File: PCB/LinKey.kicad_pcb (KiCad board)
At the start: 2 copper layers, 25 x 43.5 mm, 1 part

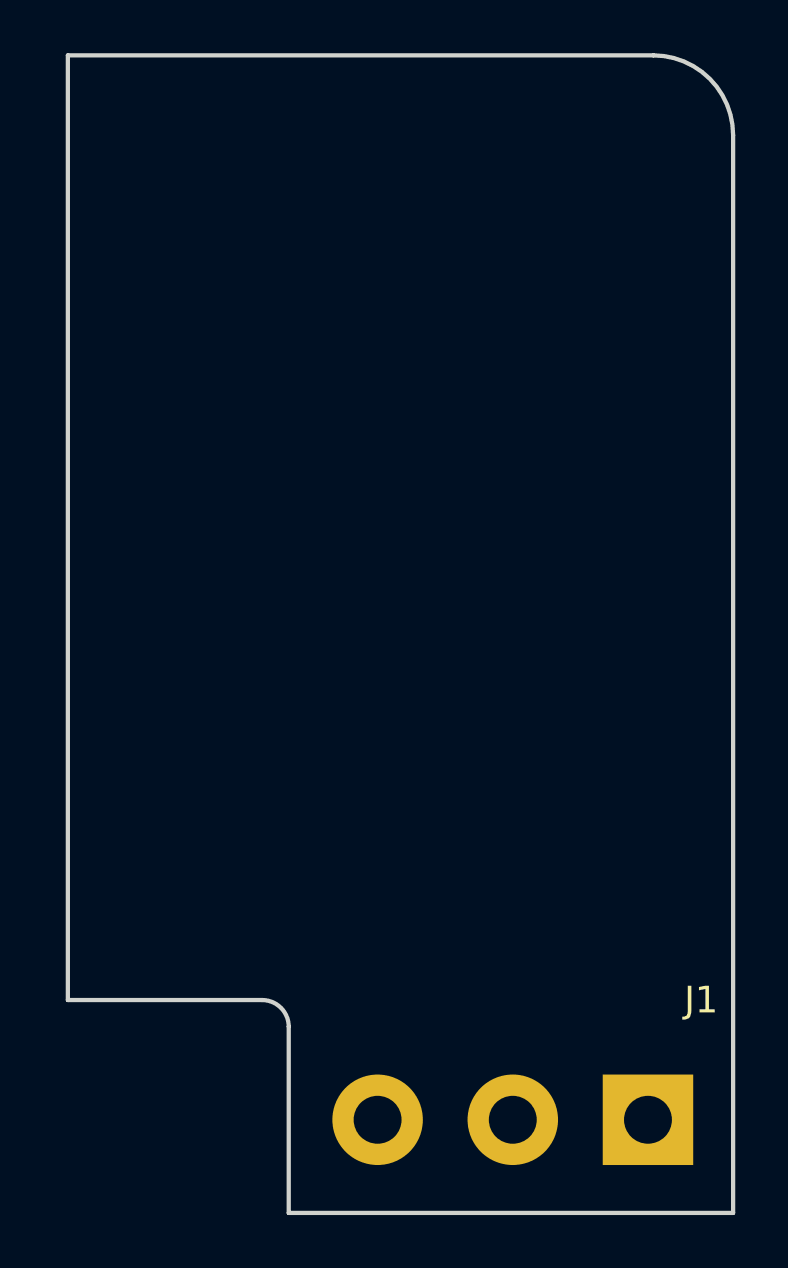
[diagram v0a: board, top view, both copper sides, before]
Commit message: Release PCB v1
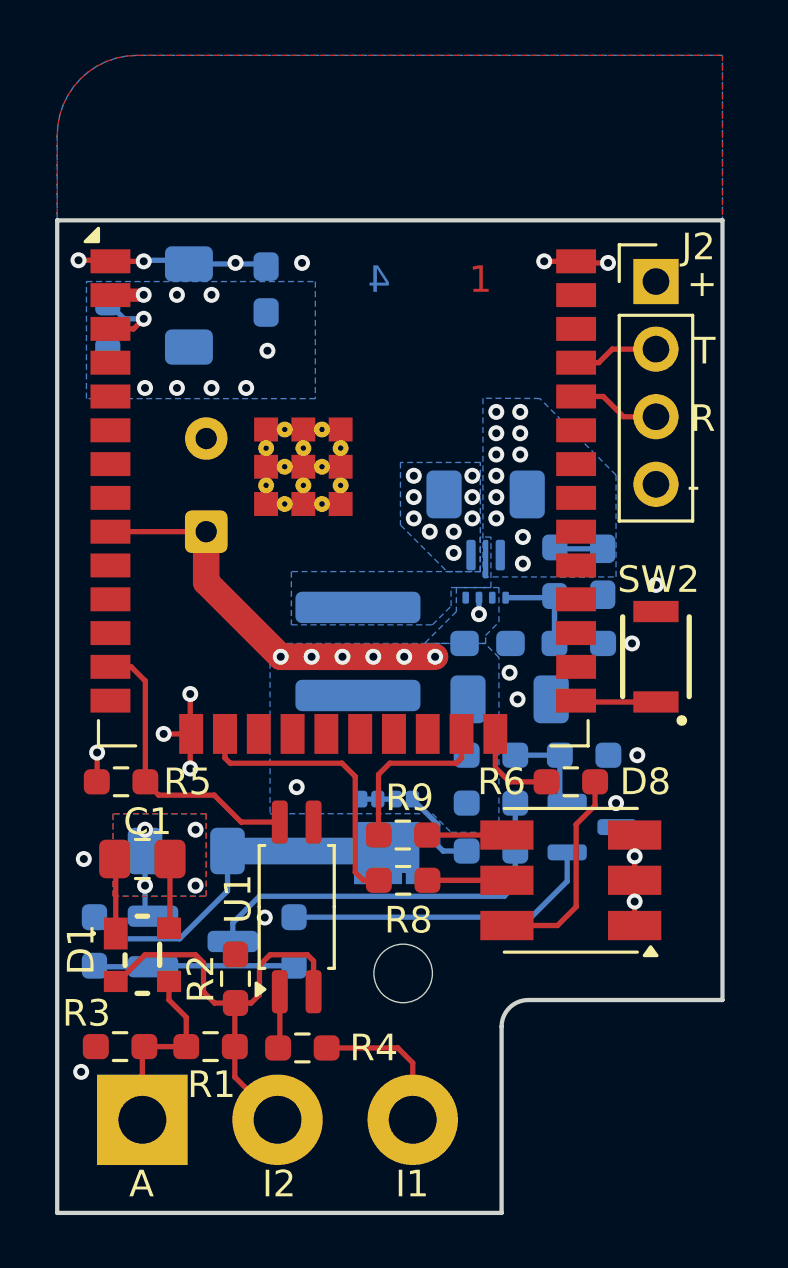
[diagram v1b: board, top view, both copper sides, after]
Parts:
- added C1: 2,2u, Capacitor_SMD:C_0805_2012Metric_Pad1.18x1.45mm_HandSolder, F.Cu at (144.5, 86.2)
- added C2: 1F, Capacitor_THT:CP_Radial_D8.0mm_P3.50mm, B.Cu at (146.9, 73.9)
- added C3: 22u, Capacitor_SMD:C_1206_3216Metric_Pad1.33x1.80mm_HandSolder, B.Cu at (158.3, 80.2)
- added C4: 100n, Capacitor_SMD:C_0603_1608Metric_Pad1.08x0.95mm_HandSolder, B.Cu at (157.5, 78.1)
- added C5: 175p, Capacitor_SMD:C_0603_1608Metric_Pad1.08x0.95mm_HandSolder, B.Cu at (161.8, 75.4)
- added C6: 22u, Capacitor_SMD:C_1206_3216Metric_Pad1.33x1.80mm_HandSolder, B.Cu at (157.4, 72.5)
- added C7: 22u, Capacitor_SMD:C_1206_3216Metric_Pad1.33x1.80mm_HandSolder, B.Cu at (146.2, 65.4)
- added C8: 100n, Capacitor_SMD:C_0603_1608Metric_Pad1.08x0.95mm_HandSolder, B.Cu at (149.2, 64.8)
- added D1: BAS_4002A_RPP_E6327, LinKey_Lib_Footprints:BAS4002ARPPE6327, F.Cu at (144.5, 89.8)
- added D8: LED_RGB, LED_SMD:LED_RGB_5050-6, F.Cu at (160.6, 87.0)
- added J2: Conn_01x04, Connector_PinHeader_2.54mm:PinHeader_1x04_P2.54mm_Vertical, F.Cu at (163.8, 64.5)
- added L1: 1uH, Inductor_SMD:L_Coilcraft_XAL5030-XXX, B.Cu at (152.6, 78.4)
- added Q1: MMBT2907ALT1G, Package_TO_SOT_SMD:SOT-23_Handsoldering, B.Cu at (146.4, 89.3)
- added Q2: CSD25402Q3A, Package_SON:VSON-8_3.3x3.3mm_P0.65mm_NexFET, B.Cu at (153.7, 85.4)
- added R1: R, Resistor_SMD:R_0603_1608Metric_Pad0.98x0.95mm_HandSolder, F.Cu at (147.1, 93.2)
- added R10: 18r, Resistor_SMD:R_1206_3216Metric_Pad1.30x1.75mm_HandSolder, B.Cu at (146.2, 85.9)
- added R11: 200r, Resistor_SMD:R_0603_1608Metric_Pad0.98x0.95mm_HandSolder, B.Cu at (142.7, 89.3)
- added R12: 120r, Resistor_SMD:R_0603_1608Metric_Pad0.98x0.95mm_HandSolder, B.Cu at (157.6, 85.9)
- added R13: 10k, Resistor_SMD:R_0603_1608Metric_Pad0.98x0.95mm_HandSolder, B.Cu at (157.6, 84.1)
- added R14: 2k, Resistor_SMD:R_0603_1608Metric_Pad0.98x0.95mm_HandSolder, B.Cu at (150.2, 89.3)
- added R15: 10k, Resistor_SMD:R_0603_1608Metric_Pad0.98x0.95mm_HandSolder, B.Cu at (157.6, 82.3)
- added R16: 100k, Resistor_SMD:R_0603_1608Metric_Pad0.98x0.95mm_HandSolder, B.Cu at (161.1, 82.3)
- added R17: 453k, Resistor_SMD:R_0603_1608Metric_Pad0.98x0.95mm_HandSolder, B.Cu at (160.0, 75.4)
- added R18: 100k, Resistor_SMD:R_0603_1608Metric_Pad0.98x0.95mm_HandSolder, B.Cu at (160.9, 78.1)
- added R2: R, Resistor_SMD:R_0603_1608Metric_Pad0.98x0.95mm_HandSolder, F.Cu at (148.0, 90.7)
- added R3: R, Resistor_SMD:R_0603_1608Metric_Pad0.98x0.95mm_HandSolder, F.Cu at (143.7, 93.2)
- added R4: 470r, Resistor_SMD:R_0603_1608Metric_Pad0.98x0.95mm_HandSolder, F.Cu at (150.5, 93.3)
- added R5: 10k, Resistor_SMD:R_0603_1608Metric_Pad0.98x0.95mm_HandSolder, F.Cu at (143.7, 83.3)
- added R6: 120r, Resistor_SMD:R_0603_1608Metric_Pad0.98x0.95mm_HandSolder, F.Cu at (160.6, 83.3)
- added R7: 10k, Resistor_SMD:R_0603_1608Metric_Pad0.98x0.95mm_HandSolder, B.Cu at (143.2, 66.2)
- added R8: 330r, Resistor_SMD:R_0603_1608Metric_Pad0.98x0.95mm_HandSolder, F.Cu at (154.3, 87.0)
- added R9: 120r, Resistor_SMD:R_0603_1608Metric_Pad0.98x0.95mm_HandSolder, F.Cu at (154.3, 85.3)
- added REF**: LayerMarker_4_6.35x2.54mm_TextH1mm_P1.27mm_BottomMirrored, Symbol:LayerMarker_4_6.35x2.54mm_TextH1mm_P1.27mm_BottomMirrored, F.Cu at (157.2, 63.2)
- added REF**: MountingHole_2.2mm_M2, MountingHole:MountingHole_2.2mm_M2, F.Cu at (154.3, 90.5)
- added SW2: ~, LinKey_Lib_Footprints:B3U-1000P, F.Cu at (163.8, 78.6)
- added U1: ACPL-214-500E, Package_SO:SOP-4_4.4x2.6mm_P1.27mm, F.Cu at (150.3, 88.0)
- added U2: ESP32-WROOM-32E, RF_Module:ESP32-WROOM-32E, F.Cu at (152.1, 69.0)
- added U4: TL431DBZ, Package_TO_SOT_SMD:SOT-23, B.Cu at (161.4, 85.0)
- added U5: TPS61022, Package_DFN_QFN:Texas_RWU0007A_VQFN-7_2x2mm_P0.5mm, B.Cu at (157.4, 75.4)
- J1: moved to B.Cu
- moved J1 19.0 mm to (144.5, 96.0), turned to 180 degrees
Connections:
- J1 pad 1: unconnected-(J1-A-Pad1) -> Net-(D1-~_2)
- J1 pad 2: unconnected-(J1-I2-Pad2) -> Net-(D1-~_1)
- J1 pad 3: unconnected-(J1-I1-Pad3) -> Net-(J1-I1)
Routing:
- net GND: track 0.00 -> 20.0 mm, vias 0 -> 31
- net Net-(D1-~_1): track 0.00 -> 17.0 mm
- net VCAP: track 0.00 -> 16.8 mm, vias 0 -> 6
- net Net-(Q1-C): track 0.00 -> 15.0 mm
- net Net-(Q2-S): track 0.00 -> 13.7 mm
- net Net-(U4-K): track 0.00 -> 11.9 mm
- net /TIC: track 0.00 -> 11.0 mm
- net /LED_RED: track 0.00 -> 10.7 mm
- net Net-(D8-RA): track 0.00 -> 7.89 mm
- net Net-(Q1-B): track 0.00 -> 7.68 mm
- net Net-(D1-~_2): track 0.00 -> 7.09 mm
- net /LED_GREEN: track 0.00 -> 6.56 mm
- net Net-(J1-I1): track 0.00 -> 5.61 mm
- net Net-(U5-FB): track 0.00 -> 5.29 mm
- net VDD: track 0.00 -> 5.20 mm, vias 0 -> 4
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- added copper zone on B.Cu, net +3.3V
- added copper zone on In2.Cu, net +3.3V
- added copper zone on B.Cu, net GND
- added copper zone on F.Cu, net GND
- added copper zone on In1.Cu, net GND
- added copper zone on B.Cu, net Net-(U5-SW)
- added copper zone on B.Cu, net VCAP
- added copper zone on B.Cu, net VDD
- added copper zone on F.Cu, net VDD
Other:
- board size 25 x 43.5 mm -> 25 x 37.3 mm
- copper layers 2 -> 4
- board text added: "+"
- board text added: "-"
- board text added: "A"
- board text added: "I1"
- board text added: "I2"
- board text added: "Linkey ESP32 01.2026 v1"
- board text added: "R"
- board text added: "T"
